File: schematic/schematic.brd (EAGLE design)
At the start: 101.3 x 80 mm, 121 parts, among them U2 ATSAM3S4AA-AU

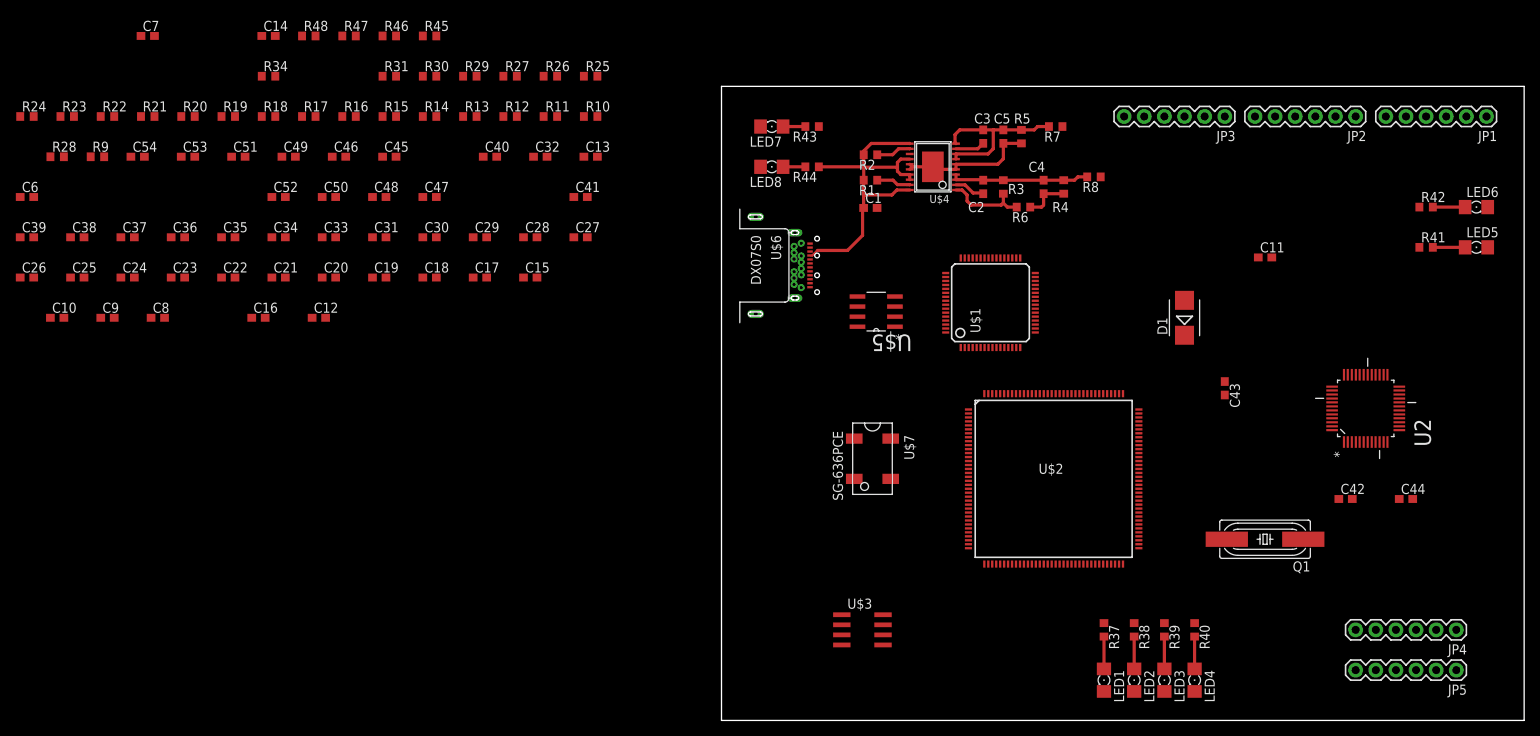
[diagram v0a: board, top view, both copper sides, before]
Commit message: Worked on BCP more.
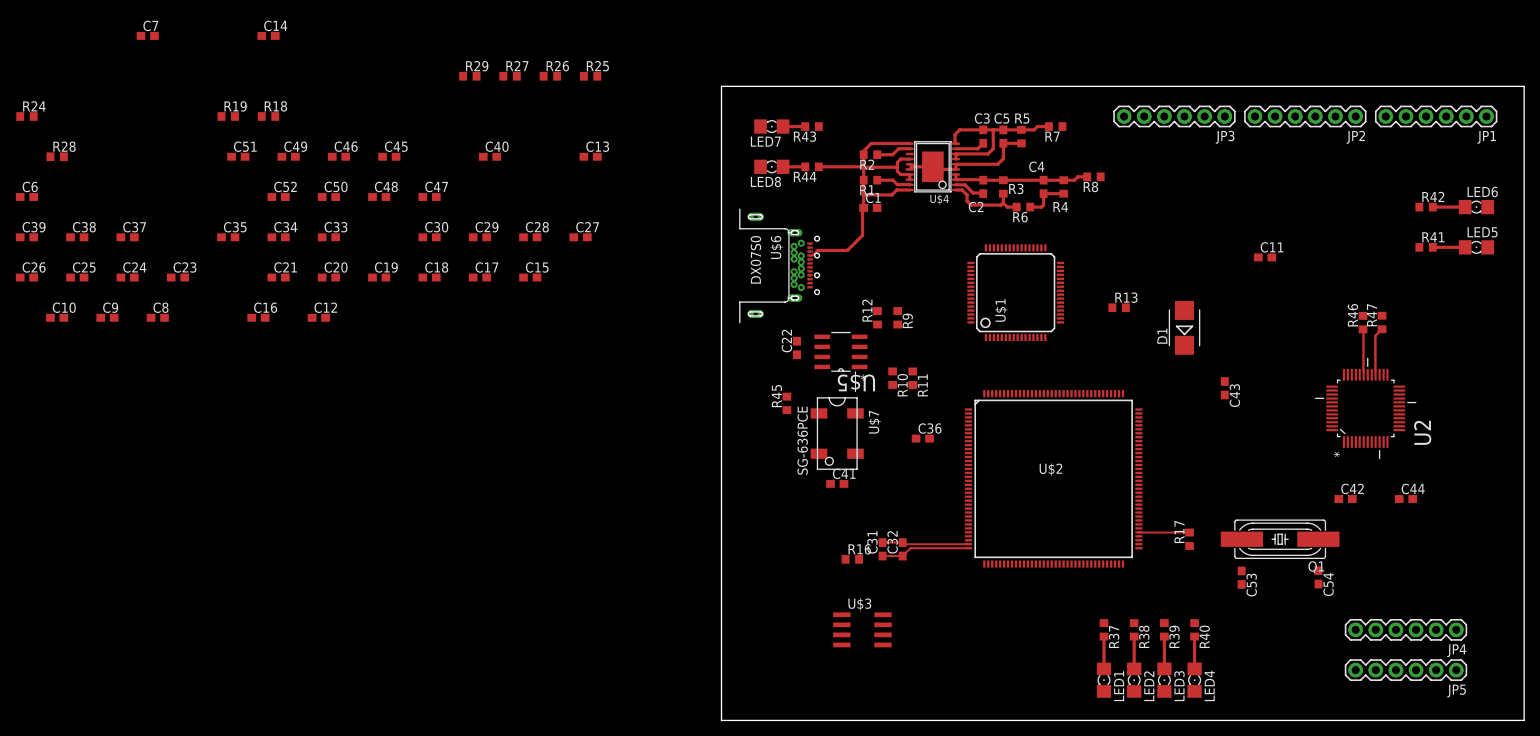
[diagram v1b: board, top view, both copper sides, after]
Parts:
- removed R14, R15, R20, R21, R22, R23, R30, R31, R34, R48: 0, resistor:R0603
- moved C54 158.2 mm to (75.3, 18.1), turned to 270 degrees
- moved C53 143.2 mm to (65.6, 18.0), turned to 270 degrees
- moved R47 135.3 mm to (83.3, 50.2), turned to 90 degrees
- moved R46 128.1 mm to (80.9, 50.2), turned to 90 degrees
- moved R17 123.3 mm to (59.1, 22.9), turned to 90 degrees
- moved R9 103.0 mm to (22.2, 50.8), turned to 270 degrees
- moved C36 97.4 mm to (25.4, 35.6)
- moved R13 85.4 mm to (50.2, 52.1)
- moved R16 84.6 mm to (16.5, 20.3)
- moved C31 74.7 mm to (20.3, 21.6), turned to 90 degrees
- moved C22 72.3 mm to (9.53, 47.0), turned to 90 degrees
- moved C32 67.4 mm to (22.9, 21.6), turned to 90 degrees
- moved R45 64.7 mm to (8.26, 40.0), turned to 90 degrees
- moved R11 56.4 mm to (24.1, 43.2), turned to 270 degrees
- moved R12 52.9 mm to (19.7, 50.8), turned to 90 degrees
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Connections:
- removed net 3.3V: C41.1, C42.1, C45.1, C46.1, C47.1, C48.1, C49.1, C50.1, C51.1, C52.1, R43.1, R45.2, R46.2, R47.2, U$7.4, U2.13, U2.33, U2.47, U2.7
- removed net N$11: R15.2, U$1.24
- removed net N$12: R23.2, U$1.16
- removed net N$13: R22.2, U$1.17
- removed net N$14: R21.2, U$1.18
- removed net N$17: R20.2, U$1.21
- removed net N$24: R30.2, U$1.38
- removed net N$25: R31.2, U$1.39
- removed net N$28: R34.2, U$1.43
- removed net N$41: R48.2, U$2.129
- removed net N$8: R14.2, U$1.23
- net +3.3V: now also C41.1, C42.1, C45.1, C46.1, C47.1, C48.1, C49.1, C50.1, C51.1, C52.1, R43.1, R45.2, R46.2, R47.2, U$7.4, U2.13, U2.33, U2.47, U2.7
- net 12MHZ: now also U$2.129; no longer R48.1
- net CDONE: now also U$1.23; no longer R14.1
- net CRESET_B: now also U$1.24; no longer R15.1
- net DTRN: now also U$1.43; no longer R34.1
- net MISO: now also U$1.18; no longer R21.1
- net MOSI: now also U$1.17; no longer R22.1
- net SCK: now also U$1.16; no longer R23.1
- net SS: now also U$1.21; no longer R20.1
- net URXD0: now also U$1.38; no longer R30.1
- net UTXD0: now also U$1.39; no longer R31.1
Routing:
- net N$15: track 0.00 -> 11.3 mm
- net N$9: track 0.00 -> 10.9 mm
- net N$16: track 0.00 -> 6.40 mm
- net TWCK0: track 0.00 -> 5.61 mm
- net TWD0: track 0.00 -> 5.30 mm
